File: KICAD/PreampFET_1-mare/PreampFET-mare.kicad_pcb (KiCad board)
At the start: 2 copper layers, 12 x 10 mm, 18 parts, among them J1 Conn_01x02, J2 Conn_01x04, Q1 JFE2140DSGR, Q2 PMP4501V_115

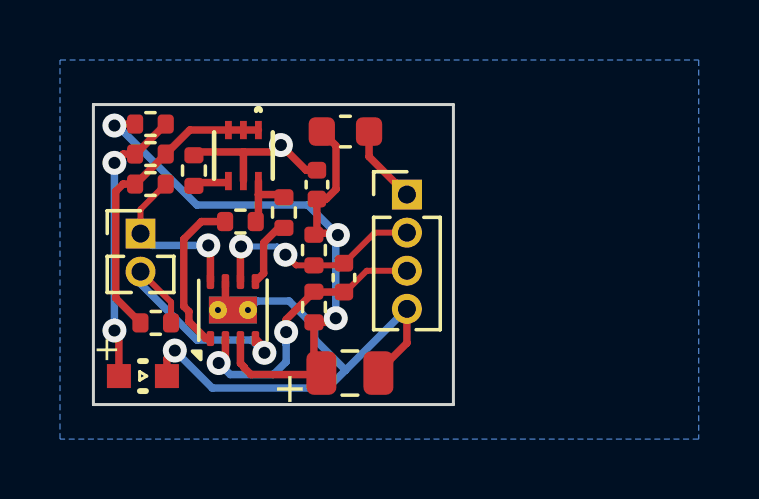
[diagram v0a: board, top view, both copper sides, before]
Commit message: v19-12-24
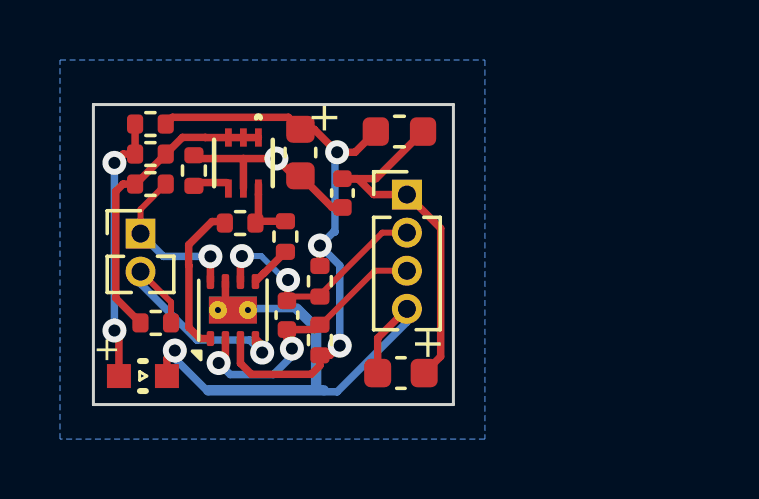
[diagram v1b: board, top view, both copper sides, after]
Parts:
- added C4: 22uF, Capacitor_SMD:C_0603_1608Metric, F.Cu at (114.5, 72.3)
- C1: value 0.1u -> 0.1uF
- C2: value 47u -> 22uF; footprint Capacitor_SMD:C_0805_2012Metric -> Capacitor_SMD:C_0603_1608Metric
- C3: value 150p -> 150pF
- R1, R3: value 10M -> 10M,1%
- R2, R4: value 1k -> 1k,0.1%
- R5, R6: value 49.9 -> 49.9,0.1%
- R7: value 360 -> 360,0.1%
- R8: value 10k -> 10k,1%
- R9: value 3.9k -> 3.9k,1%
- moved C3 2.27 mm to (114.1, 77.7)
- moved L1 1.80 mm to (117.8, 71.6), turned to 180 degrees
- moved C2 1.70 mm to (117.9, 79.7), turned to 180 degrees
- moved R2 1.12 mm to (115.2, 78.5)
- moved R4 1.06 mm to (115.2, 76.6)
- moved C1 0.89 mm to (116.0, 73.7), turned to -90 degrees
- moved R6 0.80 mm to (114.0, 75.1)
- moved Q2 0.25 mm to (112.6, 72.6)
- moved R5 0.05 mm to (112.5, 74.7)
- turned R8 to 180 degrees
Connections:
- C1 pad 1: VC -> Vcc
- C2 pad 1: VC -> Vcc
- J2 pad 1: +3V3 -> Vcc
- L1 pad 1: VC -> Vcc
- L1 pad 2: Vcc -> VC
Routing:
- net Vcc: track 0.00 -> 12.4 mm
- net VC: track 23.7 -> 20.4 mm
- net +3V3: track 2.62 -> 0.00 mm
- net GND: track 24.1 -> 26.1 mm
- net Net-(Q1-Pad5): track 2.29 -> 1.41 mm
- net /B+: track 7.42 -> 8.25 mm
